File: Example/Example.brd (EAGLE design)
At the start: 86 x 54 mm, 14 parts, among them IC1 LM555D, IC2 74LS02D, J1 UX60-MB-5S8, SW1 MFS101D-6-Z

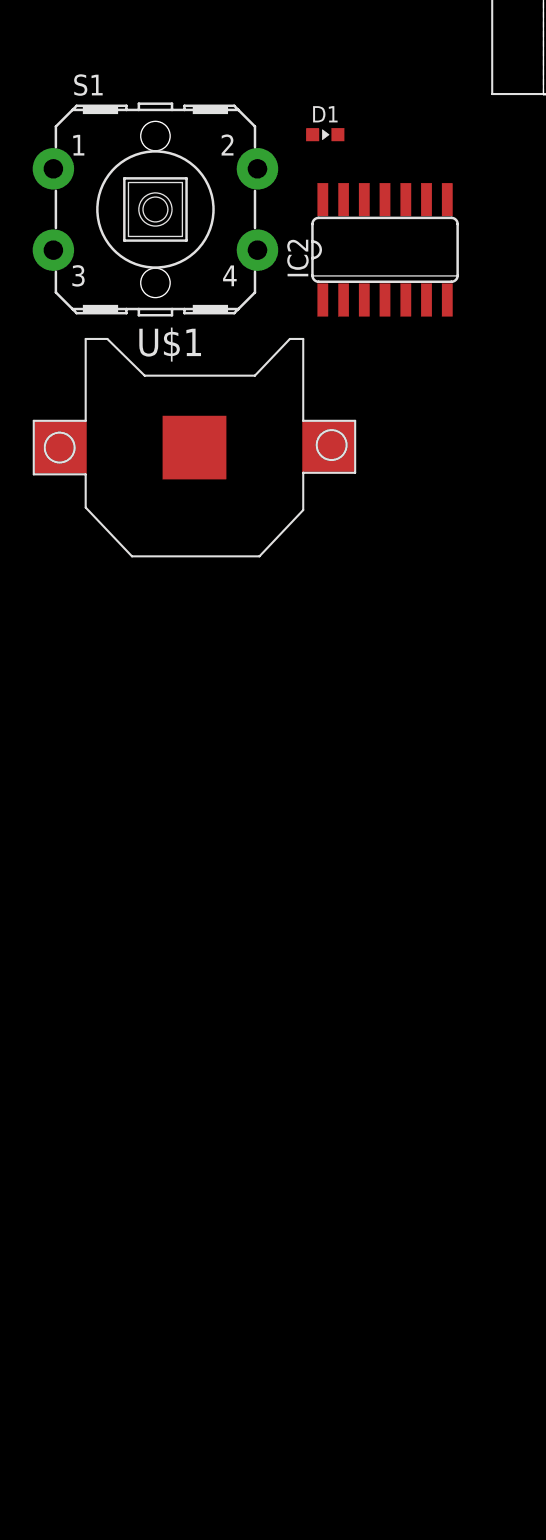
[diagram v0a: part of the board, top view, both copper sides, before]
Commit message: sr latch
finished sr latch
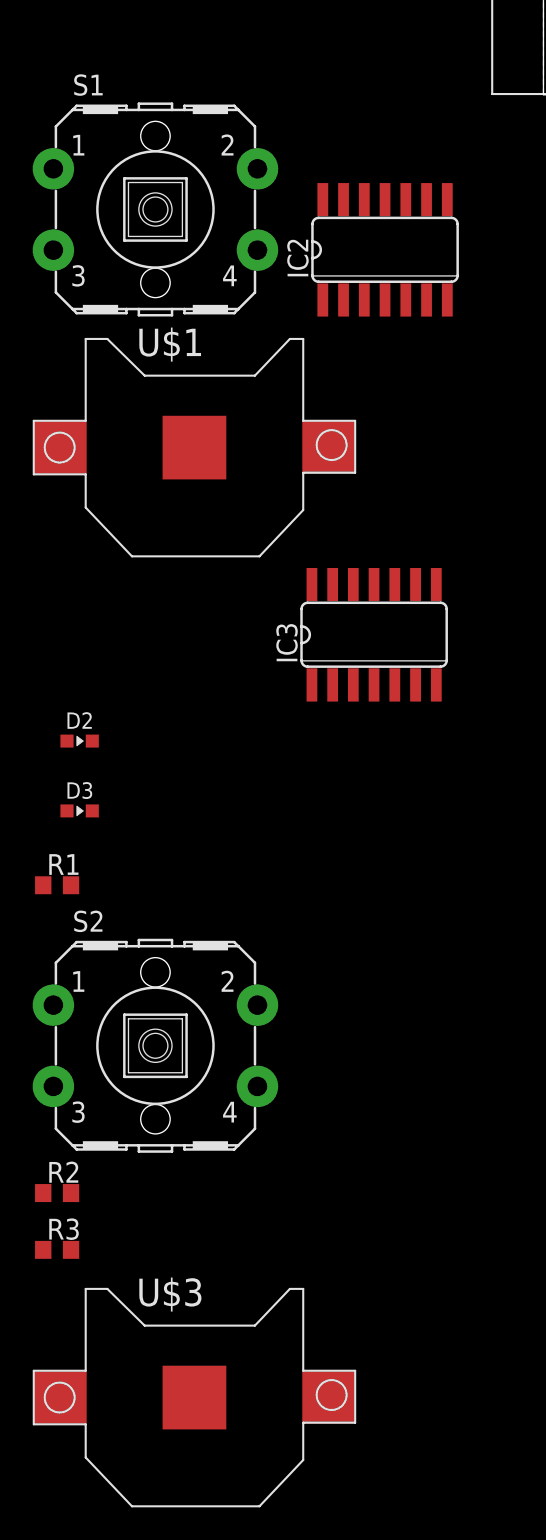
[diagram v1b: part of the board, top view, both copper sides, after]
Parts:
- removed D1: YELLOW, RoboJackets-LEDs:LED0603
- added D2, D3: YELLOW, RoboJackets-LEDs:LED0603
- added IC3: 74LS02D, 74xx-us:SO14
- added R1, R2, R3: (no value), rcl:R0603
- added S2: (no value), adafruit:B3F-40XX-ROUND
- added U$3: (no value), adafruit:CR1220-SMD
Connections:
- new net N$2: D3.A
- new net N$5: D3.C, R3.2
- new net Q: IC2.1, IC3.2
- new net QNOT: IC2.3, IC3.1
- new net R: IC2.2, R1.2, S1.2
- new net S: IC3.3, R2.2, S2.2
- net GND: now also IC3.7, R1.1, R2.1, R3.1, U$1.-, U$3.-
- net VCC: now also IC3.14, S1.3, S2.3, U$1.+$1, U$3.+$1
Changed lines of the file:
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@@
 <?xml version="1.0" encoding="utf-8"?>
 <!DOCTYPE eagle SYSTEM "eagle.dtd">
-<eagle version="9.5.2">
+<eagle version="9.5.1">
 <drawing>
 <settings>
@@
 <attribute name="DKPN" value="563-1555-ND" x="4.8" y="19.57" size="1.778" layer="27" rot="R90" display="off"/>
 </element>
-<element name="D1" library="RoboJackets-LEDs" package="LED0603" value="YELLOW" x="-13.36" y="-2.45" smashed="yes">
-<attribute name="DKPN" value="160-1448-1-ND" x="-13.36" y="-2.45" size="1.778" layer="27" display="off"/>
-<attribute name="NAME" x="-13.36" y="-1.7" size="1" layer="25" font="vector" ratio="10" align="bottom-center"/>
-<attribute name="VALUE" x="-13.36" y="-3.2" size="1" layer="27" font="vector" ratio="10" align="top-center"/>
-</element>
 <element name="IC2" library="74xx-us" library_urn="urn:adsk.eagle:library:88" package="SO14" package3d_urn="urn:adsk.eagle:package:2917/1" value="74LS02D" x="-9.7" y="-9.5" smashed="yes">
 <attribute name="NAME" x="-14.399" y="-11.278" size="1.27" layer="25" ratio="10" rot="R90"/>
@@
 <attribute name="NAME" x="-24.926" y="-16.008" size="1.6764" layer="25" font="vector"/>
 <attribute name="VALUE" x="-25.688" y="-26.16" size="1.6764" layer="27" font="vector"/>
+</element>
+<element name="IC3" library="74xx-us" library_urn="urn:adsk.eagle:library:88" package="SO14" package3d_urn="urn:adsk.eagle:package:2917/1" value="74LS02D" x="-10.37" y="-33.07" smashed="yes">
+<attribute name="NAME" x="-15.069" y="-34.848" size="1.27" layer="25" ratio="10" rot="R90"/>
+<attribute name="POPULARITY" value="0" x="-10.37" y="-33.07" size="1.778" layer="27" display="off"/>
+<attribute name="VALUE" x="-13.926" y="-33.578" size="1.27" layer="27" ratio="10"/>
+</element>
+<element name="D2" library="RoboJackets-LEDs" package="LED0603" value="YELLOW" x="-28.4" y="-39.58" smashed="yes">
+<attribute name="DKPN" value="160-1448-1-ND" x="-28.4" y="-39.58" size="1.778" layer="27" display="off"/>
+<attribute name="NAME" x="-28.4" y="-38.83" size="1" layer="25" font="vector" ratio="10" align="bottom-center"/>
+<attribute name="VALUE" x="-28.4" y="-40.33" size="1" layer="27" font="vector" ratio="10" align="top-center"/>
+</element>
+<element name="D3" library="RoboJackets-LEDs" package="LED0603" value="YELLOW" x="-28.4" y="-43.86" smashed="yes">
+<attribute name="DKPN" value="160-1448-1-ND" x="-28.4" y="-43.86" size="1.778" layer="27" display="off"/>
+<attribute name="NAME" x="-28.4" y="-43.11" size="1" layer="25" font="vector" ratio="10" align="bottom-center"/>
+<attribute name="VALUE" x="-28.4" y="-44.61" size="1" layer="27" font="vector" ratio="10" align="top-center"/>
+</element>
+<element name="R1" library="rcl" library_urn="urn:adsk.eagle:library:334" package="R0603" package3d_urn="urn:adsk.eagle:package:23555/3" value="" x="-29.78" y="-48.41" smashed="yes">
+<attribute name="NAME" x="-30.415" y="-47.775" size="1.27" layer="25"/>
+<attribute name="POPULARITY" value="77" x="-29.78" y="-48.41" size="1.778" layer="27" display="off"/>
+<attribute name="SPICEPREFIX" value="R" x="-29.78" y="-48.41" size="1.778" layer="27" display="off"/>
+<attribute name="VALUE" x="-30.415" y="-50.315" size="1.27" layer="27"/>
+</element>
+<element name="S2" library="adafruit" library_urn="urn:adsk.eagle:library:420" package="B3F-40XX-ROUND" package3d_urn="urn:adsk.eagle:package:6240926/1" value="" x="-23.76" y="-58.24" smashed="yes">
+<attribute name="NAME" x="-28.84" y="-51.255" size="1.27" layer="25" ratio="10"/>
+<attribute name="VALUE" x="-26.935" y="-63.32" size="1.27" layer="27" ratio="10"/>
+</element>
+<element name="R2" library="rcl" library_urn="urn:adsk.eagle:library:334" package="R0603" package3d_urn="urn:adsk.eagle:package:23555/3" value="" x="-29.78" y="-67.26" smashed="yes">
+<attribute name="NAME" x="-30.415" y="-66.625" size="1.27" layer="25"/>
+<attribute name="POPULARITY" value="77" x="-44.82" y="-51.89" size="1.778" layer="27" display="off"/>
+<attribute name="SPICEPREFIX" value="R" x="-44.82" y="-51.89" size="1.778" layer="27" display="off"/>
+<attribute name="VALUE" x="-30.415" y="-69.165" size="1.27" layer="27"/>
+</element>
+<element name="R3" library="rcl" library_urn="urn:adsk.eagle:library:334" package="R0603" package3d_urn="urn:adsk.eagle:package:23555/3" value="" x="-29.78" y="-70.74" smashed="yes">
+<attribute name="NAME" x="-30.415" y="-70.105" size="1.27" layer="25"/>
+<attribute name="POPULARITY" value="77" x="-29.78" y="-70.74" size="1.778" layer="27" display="off"/>
+<attribute name="SPICEPREFIX" value="R" x="-29.78" y="-70.74" size="1.778" layer="27" display="off"/>
+<attribute name="VALUE" x="-30.415" y="-72.645" size="1.27" layer="27"/>
+</element>
+<element name="U$3" library="adafruit" library_urn="urn:adsk.eagle:library:420" package="CR1220-SMD" package3d_urn="urn:adsk.eagle:package:6240665/1" value="" x="-21.37" y="-79.78" smashed="yes">
+<attribute name="NAME" x="-24.926" y="-74.178" size="1.6764" layer="25" font="vector"/>
+<attribute name="VALUE" x="-25.688" y="-84.33" size="1.6764" layer="27" font="vector"/>
 </element>
 </elements>
@@
 <via x="16.17" y="13.49" extent="1-16" drill="0.35"/>
 <contactref element="IC2" pad="7"/>
-<wire x1="10.06" y1="24.08" x2="9.58" y2="32.46" width="0" layer="19" extent="1-1"/>
-<wire x1="13.11" y1="24.29" x2="11.5" y2="23.43" width="0" layer="19" extent="1-1"/>
-<wire x1="20.2944" y1="15.719" x2="14.546" y2="23.495" width="0" layer="19" extent="1-1"/>
-<wire x1="16.17" y1="13.49" x2="20.2944" y2="15.719" width="0" layer="19" extent="1-1"/>
-<wire x1="14.105" y1="11.66" x2="14.105" y2="13.783" width="0" layer="19" extent="1-1"/>
-<wire x1="4.562" y1="4.54" x2="13.54" y2="9.9" width="0" layer="19" extent="1-1"/>
-<wire x1="-5.89" y1="-12.5734" x2="4.562" y2="4.54" width="0" layer="19" extent="1-1"/>
+<contactref element="IC3" pad="7"/>
+<contactref element="R1" pad="1"/>
+<contactref element="R2" pad="1"/>
+<contactref element="R3" pad="1"/>
+<contactref element="U$1" pad="-"/>
+<contactref element="U$3" pad="-"/>
+<wire x1="-30.63" y1="-67.26" x2="-30.63" y2="-70.74" width="0" layer="19" extent="1-1"/>
+<wire x1="-21.37" y1="-79.78" x2="-30.63" y2="-70.74" width="0" layer="19" extent="1-1"/>
+<wire x1="-30.63" y1="-48.41" x2="-30.63" y2="-67.26" width="0" layer="19" extent="1-1"/>
+<wire x1="-6.56" y1="-36.1434" x2="-30.63" y2="-48.41" width="0" layer="19" extent="1-1"/>
+<wire x1="-21.37" y1="-21.61" x2="-6.56" y2="-36.1434" width="0" layer="19" extent="1-1"/>
+<wire x1="-5.89" y1="-12.5734" x2="-21.37" y2="-21.61" width="0" layer="19" extent="1-1"/>
+<wire x1="4.562" y1="4.54" x2="-5.89" y2="-12.5734" width="0" layer="19" extent="1-1"/>
+<wire x1="13.54" y1="9.9" x2="4.562" y2="4.54" width="0" layer="19" extent="1-1"/>
+<wire x1="14.105" y1="13.783" x2="14.105" y2="11.66" width="0" layer="19" extent="1-1"/>
+<wire x1="20.2944" y1="15.719" x2="16.17" y2="13.49" width="0" layer="19" extent="1-1"/>
+<wire x1="14.546" y1="23.495" x2="20.2944" y2="15.719" width="0" layer="19" extent="1-1"/>
+<wire x1="11.5" y1="23.43" x2="13.11" y2="24.29" width="0" layer="19" extent="1-1"/>
+<wire x1="9.58" y1="32.46" x2="10.06" y2="24.08" width="0" layer="19" extent="1-1"/>
 </signal>
 <signal name="+9V">
@@
 <signal name="VCC">
 <contactref element="IC2" pad="14"/>
+<contactref element="IC3" pad="14"/>
+<contactref element="S1" pad="3"/>
+<contactref element="S2" pad="3"/>
+<contactref element="U$1" pad="+$1"/>
+<contactref element="U$3" pad="+$1"/>
+<wire x1="-30.0084" y1="-60.7292" x2="-29.57" y2="-79.78" width="0" layer="19" extent="1-1"/>
+<wire x1="-14.18" y1="-29.9966" x2="-30.0084" y2="-60.7292" width="0" layer="19" extent="1-1"/>
+<wire x1="-29.57" y1="-21.61" x2="-14.18" y2="-29.9966" width="0" layer="19" extent="1-1"/>
+<wire x1="-30.0084" y1="-9.5192" x2="-29.57" y2="-21.61" width="0" layer="19" extent="1-1"/>
+<wire x1="-13.51" y1="-6.4266" x2="-30.0084" y2="-9.5192" width="0" layer="19" extent="1-1"/>
+</signal>
+<signal name="QNOT">
+<contactref element="IC2" pad="3"/>
+<contactref element="IC3" pad="1"/>
+<wire x1="-10.97" y1="-12.5734" x2="-14.18" y2="-36.1434" width="0" layer="19" extent="1-1"/>
+</signal>
+<signal name="R">
+<contactref element="IC2" pad="2"/>
+<contactref element="S1" pad="2"/>
+<contactref element="R1" pad="2"/>
+<wire x1="-12.24" y1="-12.5734" x2="-28.93" y2="-48.41" width="0" layer="19" extent="1-1"/>
+<wire x1="-17.5116" y1="-4.5408" x2="-12.24" y2="-12.5734" width="0" layer="19" extent="1-1"/>
+</signal>
+<signal name="Q">
+<contactref element="IC3" pad="2"/>
+<contactref element="IC2" pad="1"/>
+<wire x1="-13.51" y1="-12.5734" x2="-12.91" y2="-36.1434" width="0" layer="19" extent="1-1"/>
+</signal>
+<signal name="S">
+<contactref element="IC3" pad="3"/>
+<contactref element="S2" pad="2"/>
+<contactref element="R2" pad="2"/>
+<wire x1="-17.5116" y1="-55.7508" x2="-28.93" y2="-67.26" width="0" layer="19" extent="1-1"/>
+<wire x1="-11.64" y1="-36.1434" x2="-17.5116" y2="-55.7508" width="0" layer="19" extent="1-1"/>
+</signal>
+<signal name="N$2">
+<contactref element="D3" pad="A"/>
+</signal>
+<signal name="N$5">
+<contactref element="D3" pad="C"/>
+<contactref element="R3" pad="2"/>
+<wire x1="-27.625" y1="-43.86" x2="-28.93" y2="-70.74" width="0" layer="19" extent="1-1"/>
 </signal>
 </signals>
